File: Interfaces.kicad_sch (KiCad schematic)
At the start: 8 parts, among them J6 Conn_01x04, J7 200528-0100

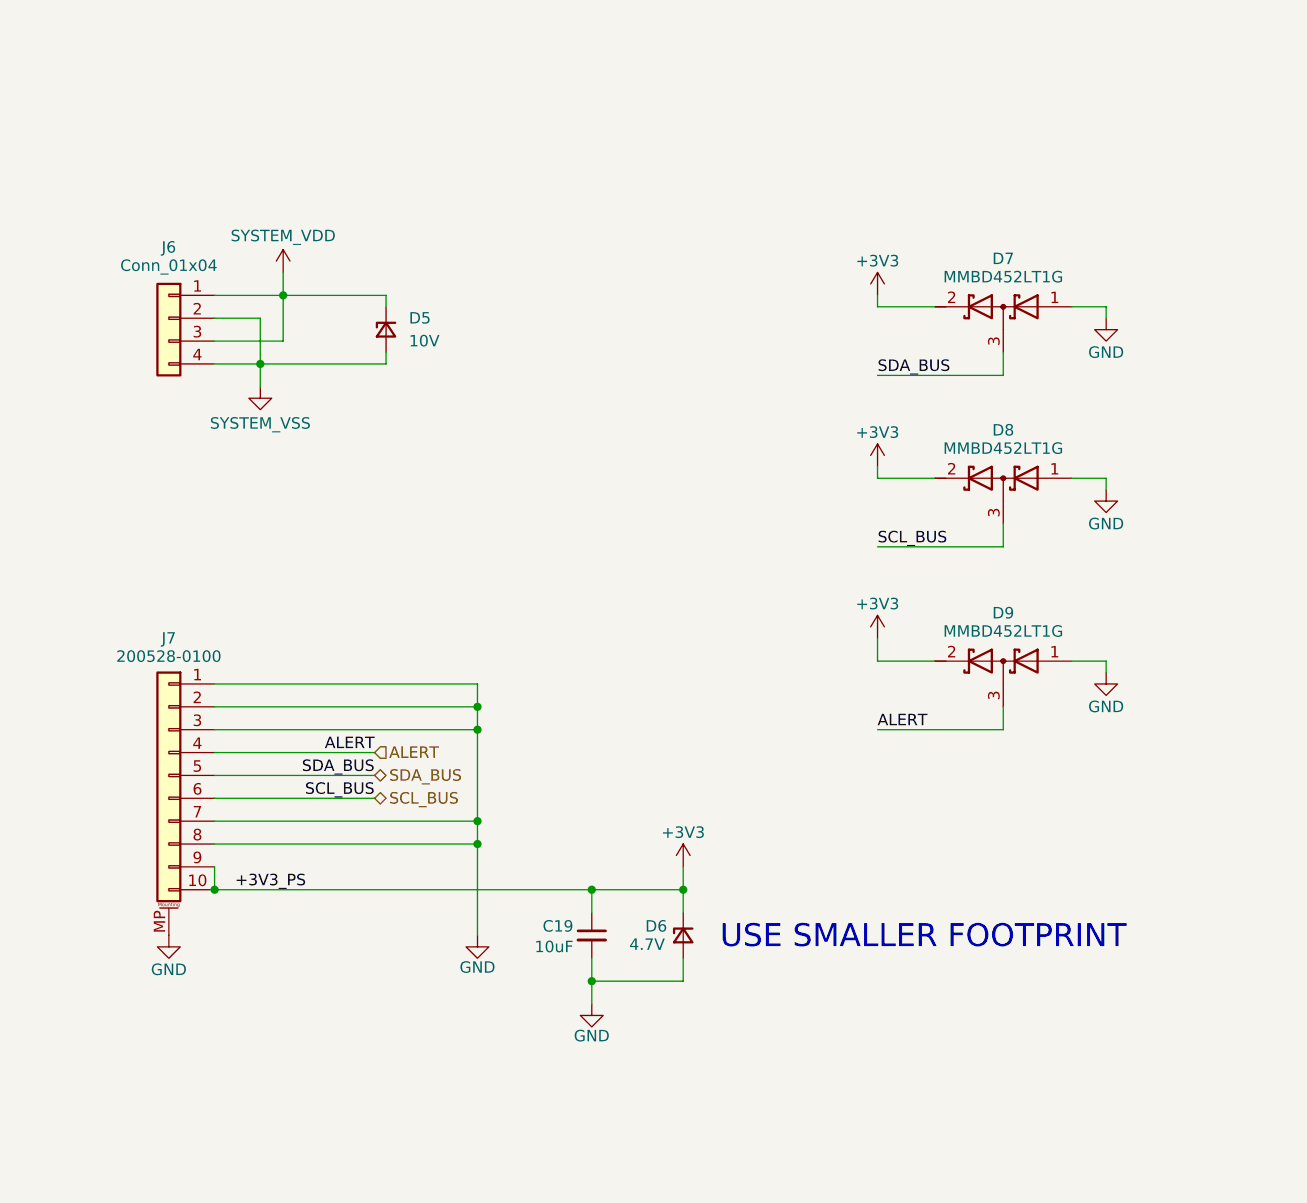
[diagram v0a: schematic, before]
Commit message: More updates
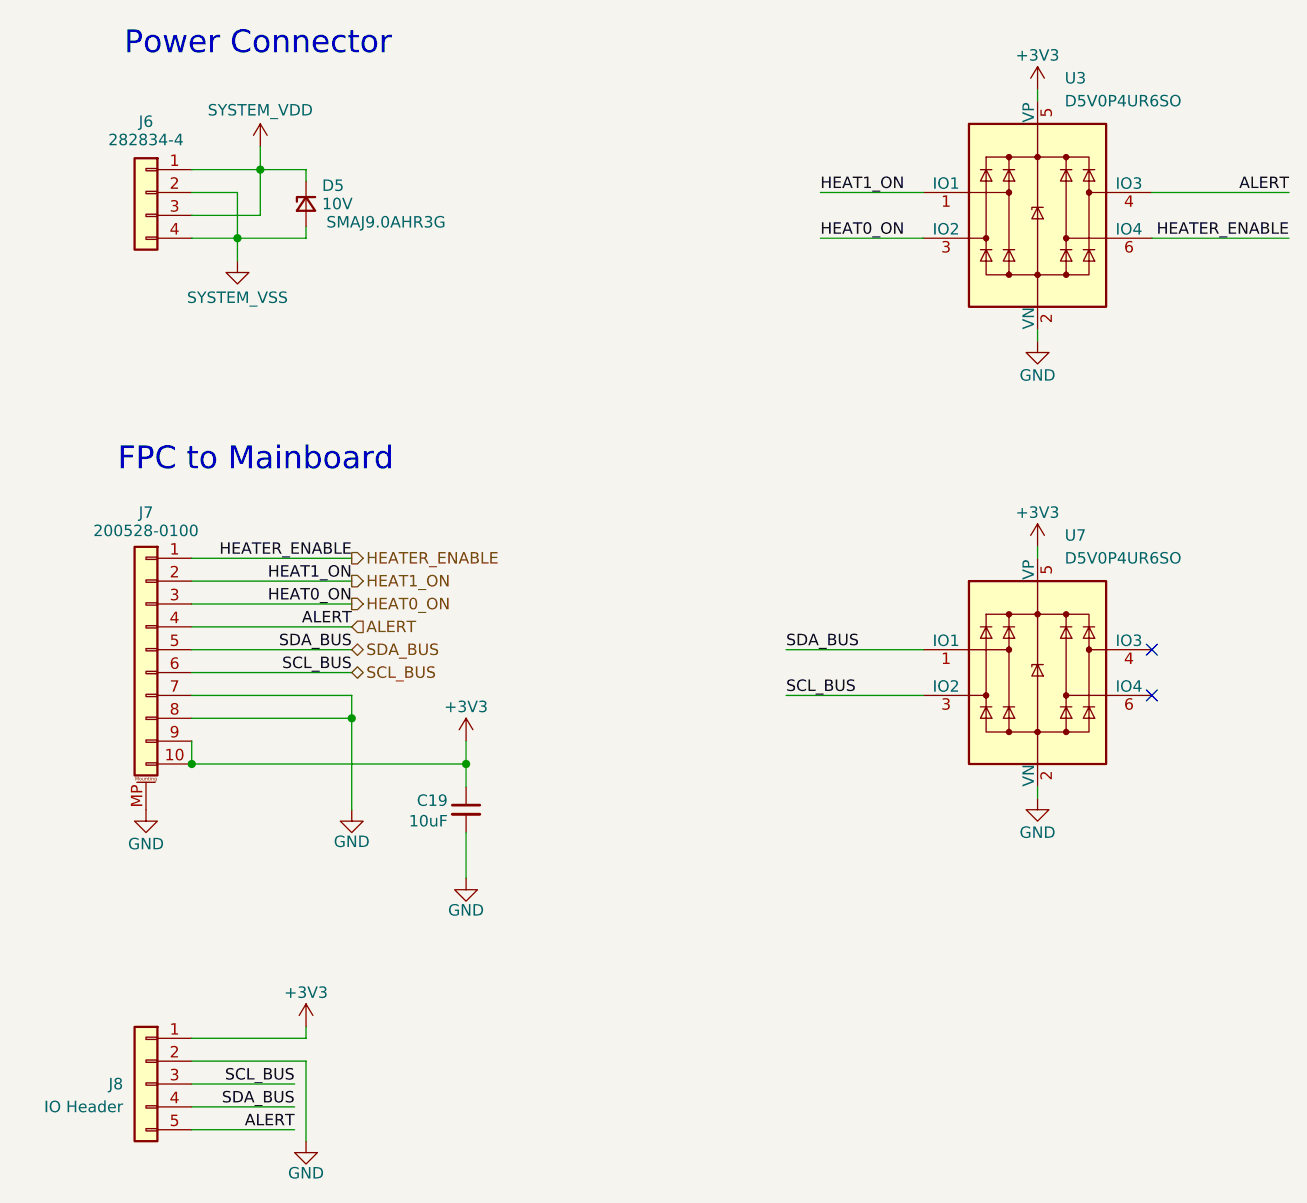
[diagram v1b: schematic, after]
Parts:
- removed D6: 4.7V, Diode_SMD:D_SMA, symbol Device:D_Zener_Small
- removed D7, D8, D9: MMBD452LT1G, Package_TO_SOT_SMD:SOT-23-3, symbol Device:D_Schottky_Dual_Series_AKC
- added J8: IO Header, Connector_PinHeader_2.54mm:PinHeader_1x05_P2.54mm_Vertical_SMD_Pin1Left, symbol Connector_Generic:Conn_01x05
- added U3, U7: D5V0P4UR6SO, Package_TO_SOT_SMD:SOT-23-6, symbol Power_Protection:SRV05-4
- D5: Part (none) -> SMAJ9.0AHR3G
- J6: value Conn_01x04 -> 282834-4; footprint (none) -> TerminalBlock_TE-Connectivity:TerminalBlock_TE_282834-4_1x04_P2.54mm_Horizontal
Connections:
- net +3V3: now also J8.1 (Pin_1), U3.5 (VP), U7.5 (VP)
- net ALERT: now also J8.5 (Pin_5), U3.4 (IO3)
- net GND: now also J8.2 (Pin_2), U3.2 (VN), U7.2 (VN); no longer J7.1 (Pin_1), J7.2 (Pin_2), J7.3 (Pin_3)
- net SCL_BUS: now also J8.3 (Pin_3), U7.3 (IO2)
- net SDA_BUS: now also J8.4 (Pin_4), U7.1 (IO1)
- new net HEAT0_ON: J7.3 (Pin_3), U3.3 (IO2)
- new net HEAT1_ON: J7.2 (Pin_2), U3.1 (IO1)
- new net HEATER_ENABLE: J7.1 (Pin_1), U3.6 (IO4)
- no-connect marks 0 -> 2
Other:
- note added: "FPC to Mainboard"
- note added: "Power Connector"
- note removed: "USE SMALLER FOOTPRINT"
- moved on the sheet: C19, D5, J6, J7
